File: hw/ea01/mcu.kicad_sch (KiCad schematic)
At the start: 46 parts, among them J2 USB_B, J3 Conn_01x05_Pin, J8 Conn_01x03_Pin, J9 Conn_01x03_Pin, SW1 SW_Push, SW2 SW_Push, U1 RP2040, U11 W25Q32JVSS, Y1 12Mhz

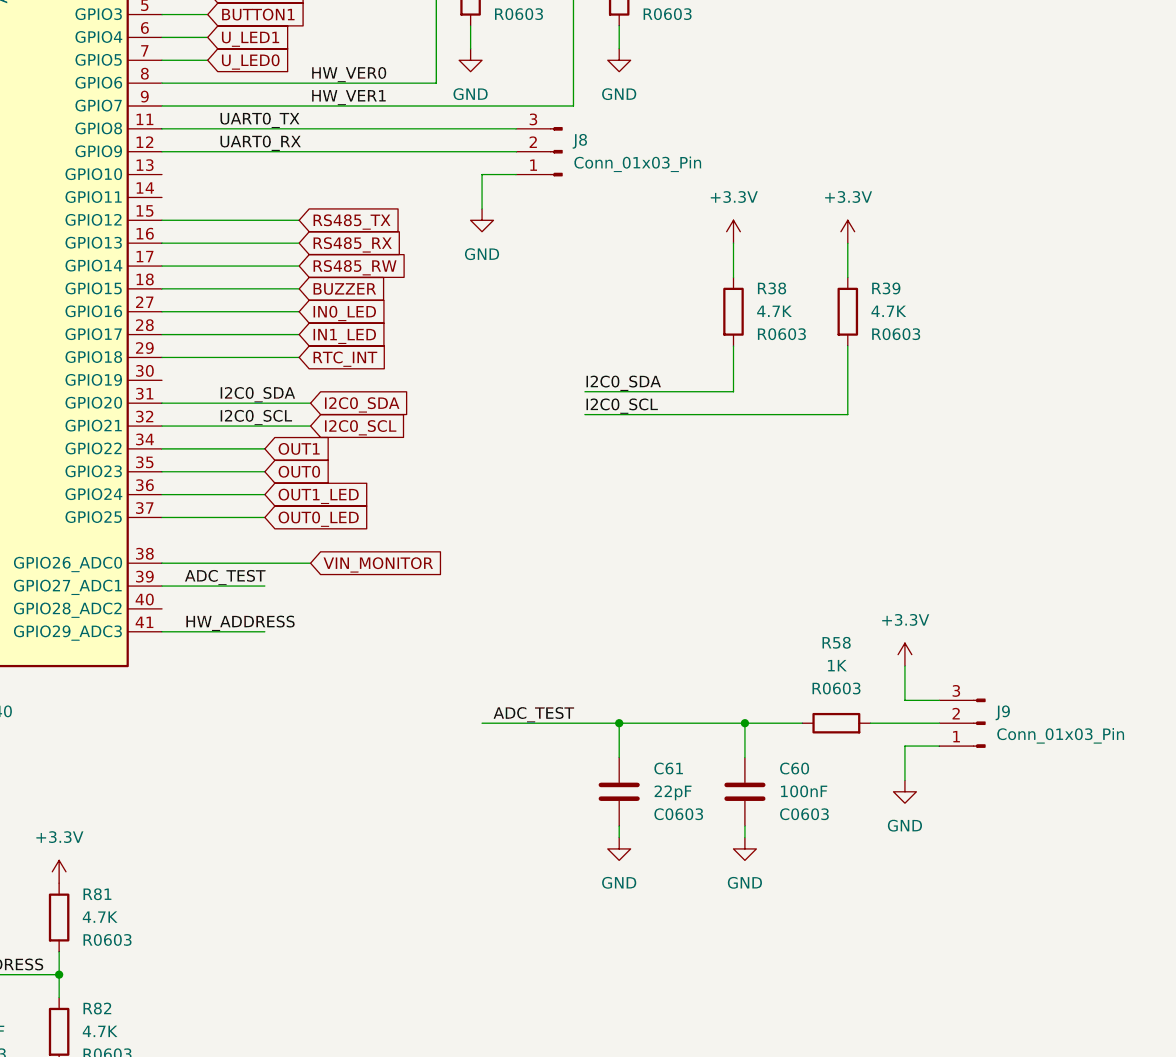
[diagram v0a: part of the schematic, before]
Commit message: drawing continue...
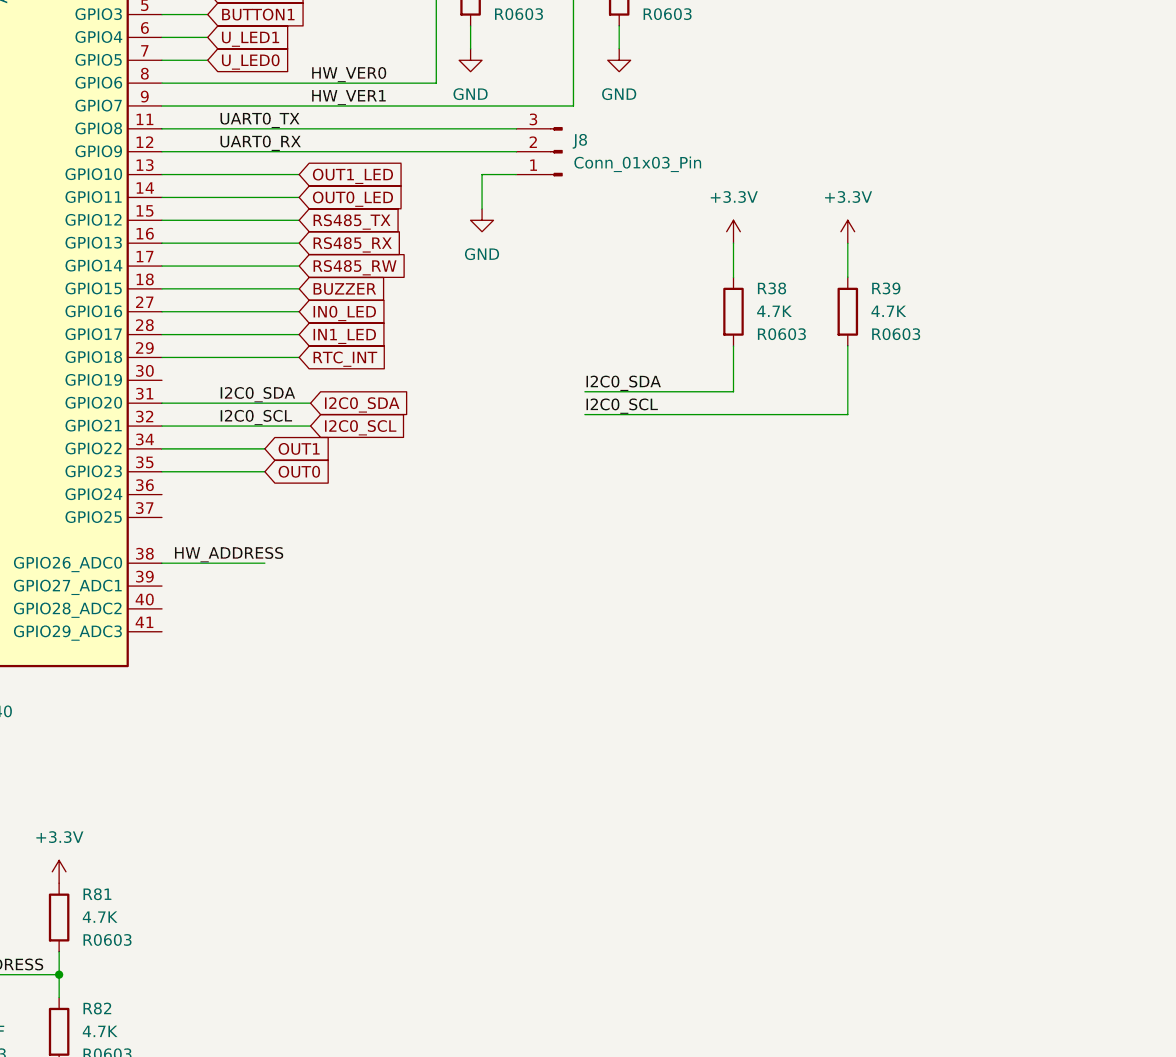
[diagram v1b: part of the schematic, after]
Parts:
- removed C60: 100nF, Capacitor_SMD:C_0603_1608Metric, symbol Device:C
- removed C61: 22pF, Capacitor_SMD:C_0603_1608Metric, symbol Device:C
- removed J9: Conn_01x03_Pin, Connector_PinHeader_2.54mm:PinHeader_1x03_P2.54mm_Vertical, symbol Connector:Conn_01x03_Pin
- removed R58: 1K, Resistor_SMD:R_0603_1608Metric, symbol Device:R
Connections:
- net VIN_MONITOR is gone; now on net HW_ADDRESS: U1.38 (GPIO26_ADC0)
- net HW_ADDRESS: no longer U1.41 (GPIO29_ADC3)
- net OUT0_LED: now also U1.14 (GPIO11); no longer U1.37 (GPIO25)
- net OUT1_LED: now also U1.13 (GPIO10); no longer U1.36 (GPIO24)
- net ADC_TEST: no longer names the net of U1.39 (GPIO27_ADC1)

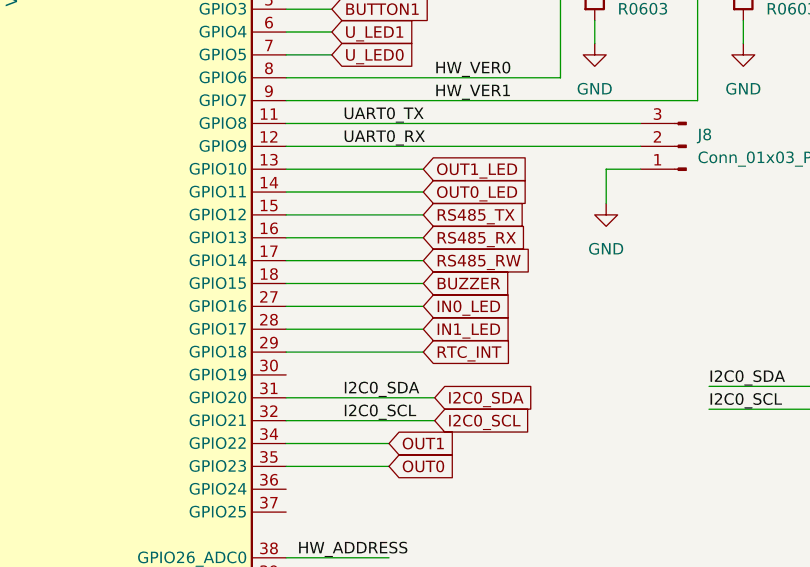
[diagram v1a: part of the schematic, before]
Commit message: drawing continue..
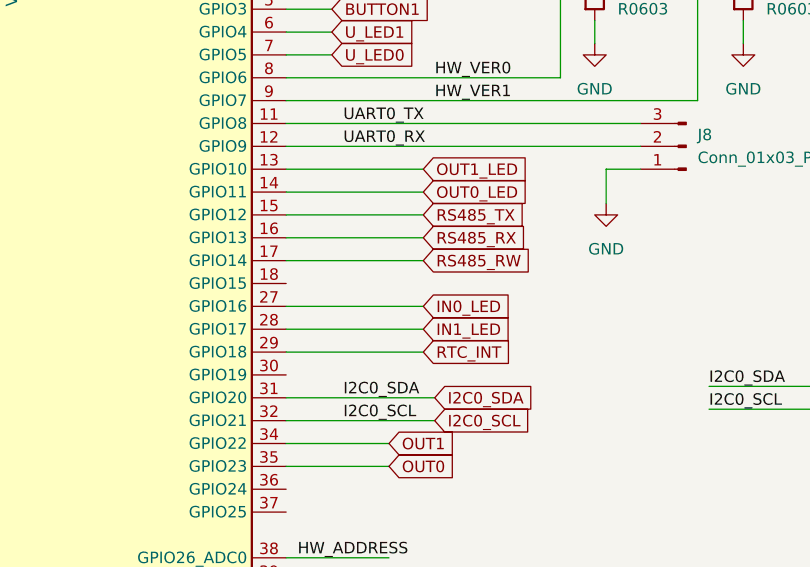
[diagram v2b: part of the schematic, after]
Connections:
- net BUZZER: no longer names the net of U1.18 (GPIO15)
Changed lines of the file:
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@@
-	(wire
-		(pts
-			(xy 172.72 95.25) (xy 187.96 95.25)
-		)
-		(stroke
-			(width 0)
-			(type default)
-		)
-	)
 	(wire
 		(pts
@@
 			(effects
 				(font
-					(size 1.27 1.27)
-				)
-				(justify left)
-				(hide yes)
-			)
-		)
-	)
-	(global_label "BUZZER"
-		(shape input)
-		(at 187.96 95.25 0)
-		(fields_autoplaced yes)
-		(effects
-			(font
-				(size 1.27 1.27)
-			)
-			(justify left)
-		)
-		(property "Intersheetrefs" "${INTERSHEET_REFS}"
-			(at 198.3837 95.25 0)
-			(effects
-				(font
